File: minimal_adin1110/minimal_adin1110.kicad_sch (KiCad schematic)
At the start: 71 parts, among them J1 CLP-114-02-G-D-BE, J2 CLP-102-02-G-D-BE, J3 CLP-102-02-G-D-BE, J4 CLP-102-02-G-D-BE, J5 CLP-103-02-G-D-BE, U1 ADIN1110CCPZ, Y1 25.0000MHz

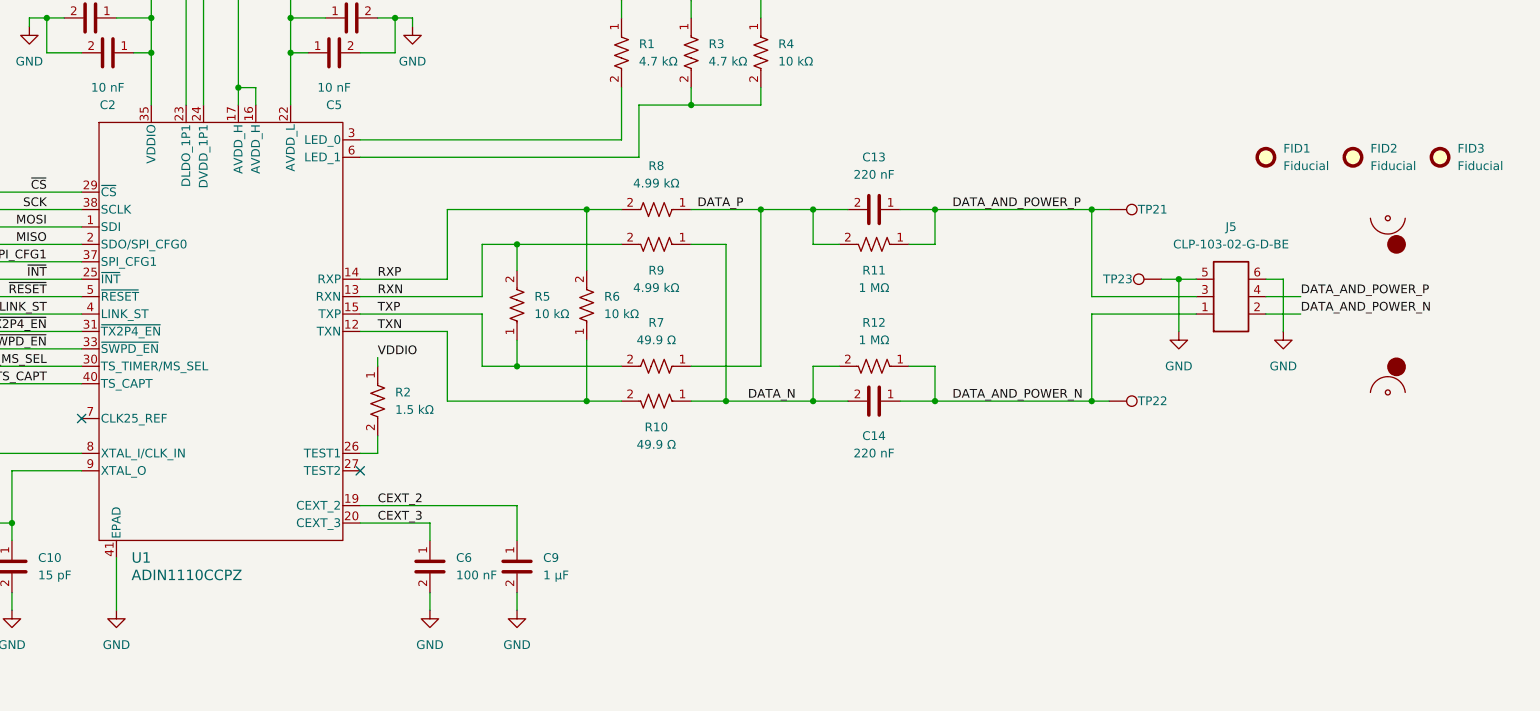
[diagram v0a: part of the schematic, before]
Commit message: Update subproject commit for KiCAD Symbol Generator
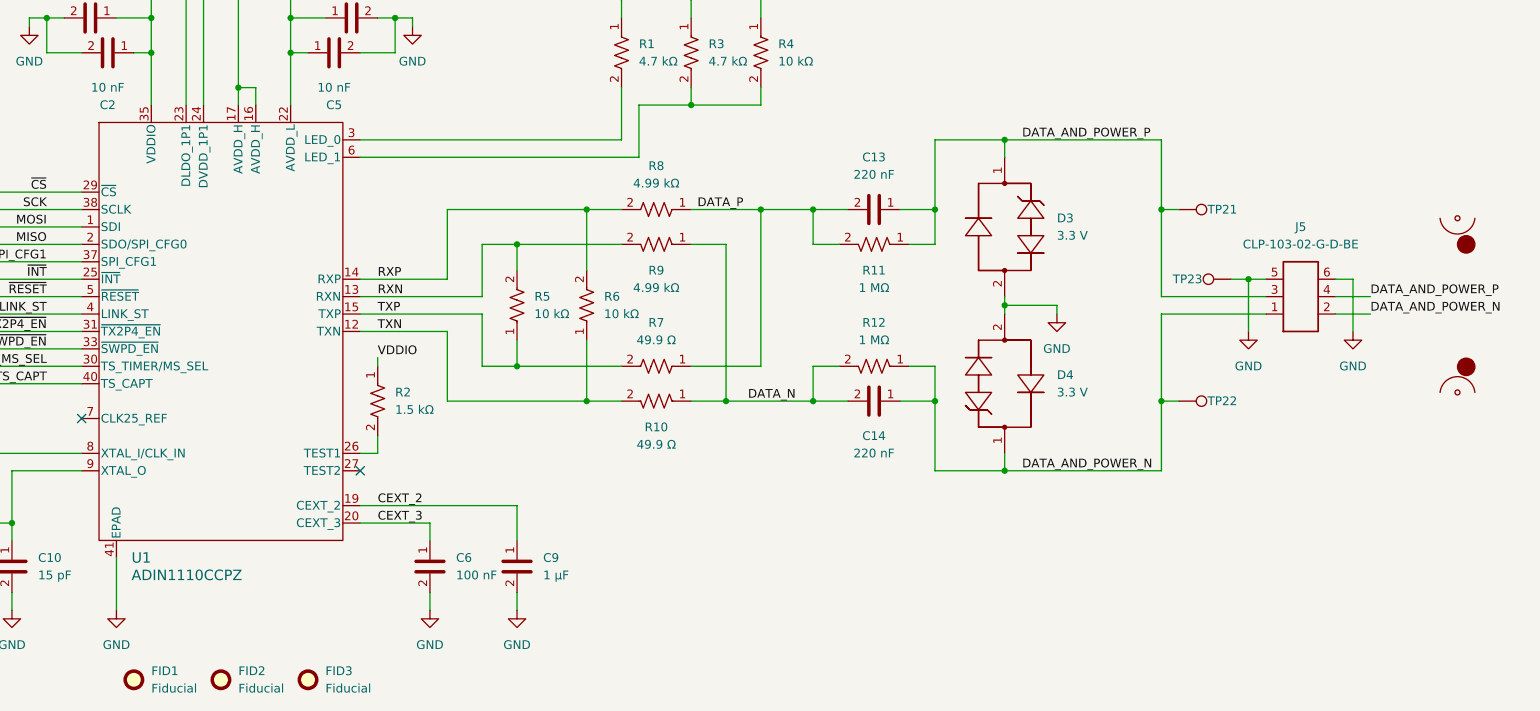
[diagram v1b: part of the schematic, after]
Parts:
- added D3, D4: 3.3 V, diode_footprints:SOD323, symbol UNITED_DIODES_DATA_BASE:D_SP4020-01FTG
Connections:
- net DATA_AND_POWER_N: now also D4.1
- net DATA_AND_POWER_P: now also D3.1
- net GND: now also D3.2, D4.2
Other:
- moved on the sheet: FID1, FID2, FID3, J5, TP21, TP22, TP23
